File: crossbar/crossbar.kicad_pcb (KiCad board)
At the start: 2 copper layers, 57.2 x 57.2 mm, 22 parts, among them J1 Conn_01x16_Pin, J10 Conn_01x16_Pin, J11 Conn_01x16_Pin, J12 Conn_01x16_Pin, J13 Conn_01x16_Pin, J14 Conn_01x16_Pin, J15 Conn_01x16_Pin, J16 Conn_01x16_Pin, J17 Conn_01x16_Pin, J18 Conn_01x16_Pin, J19 Conn_01x04_Pin, J2 Conn_01x16_Socket, J20 Conn_01x04_Pin, J21 Conn_01x04_Socket, J22 Conn_01x04_Socket, J3 Conn_01x16_Pin, J4 Conn_01x16_Pin, J5 Conn_01x16_Pin, J6 Conn_01x16_Pin, J7 Conn_01x16_Pin, J8 Conn_01x16_Pin, J9 Conn_01x16_Pin

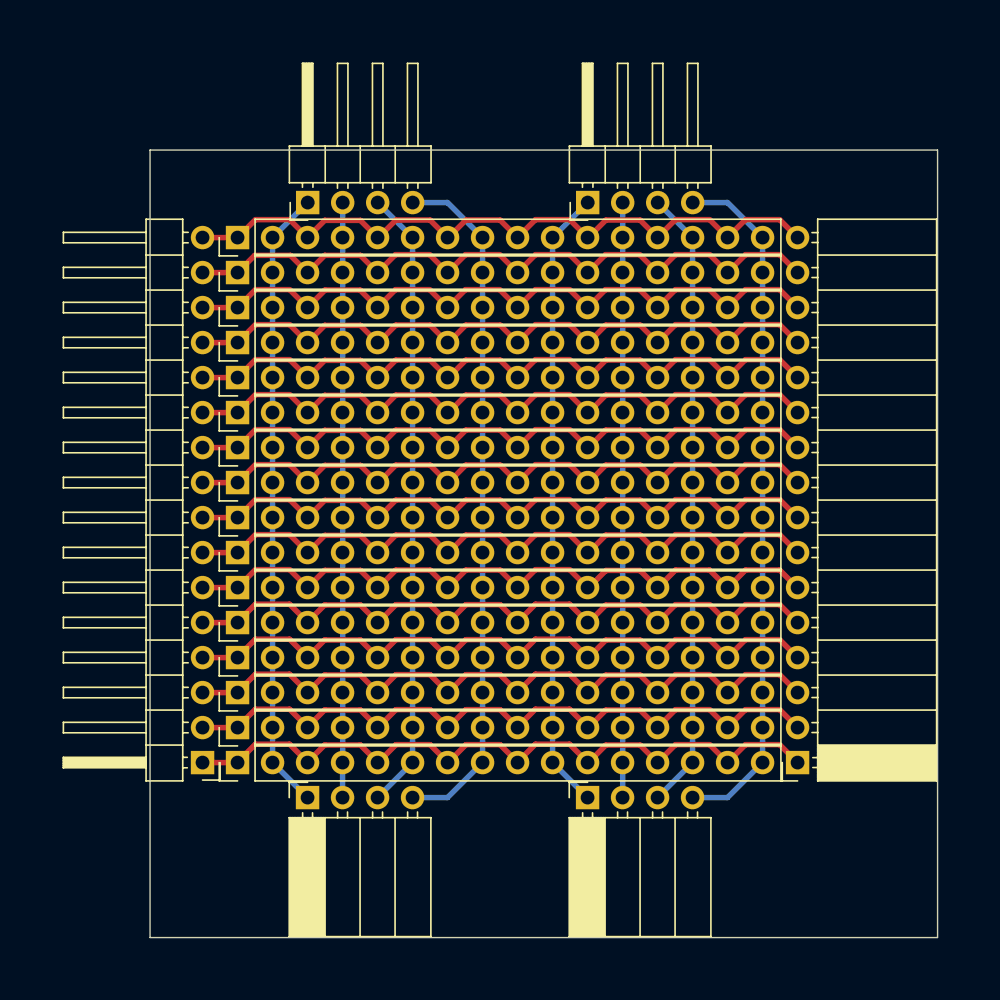
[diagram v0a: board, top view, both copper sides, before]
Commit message: crossbar & terminals
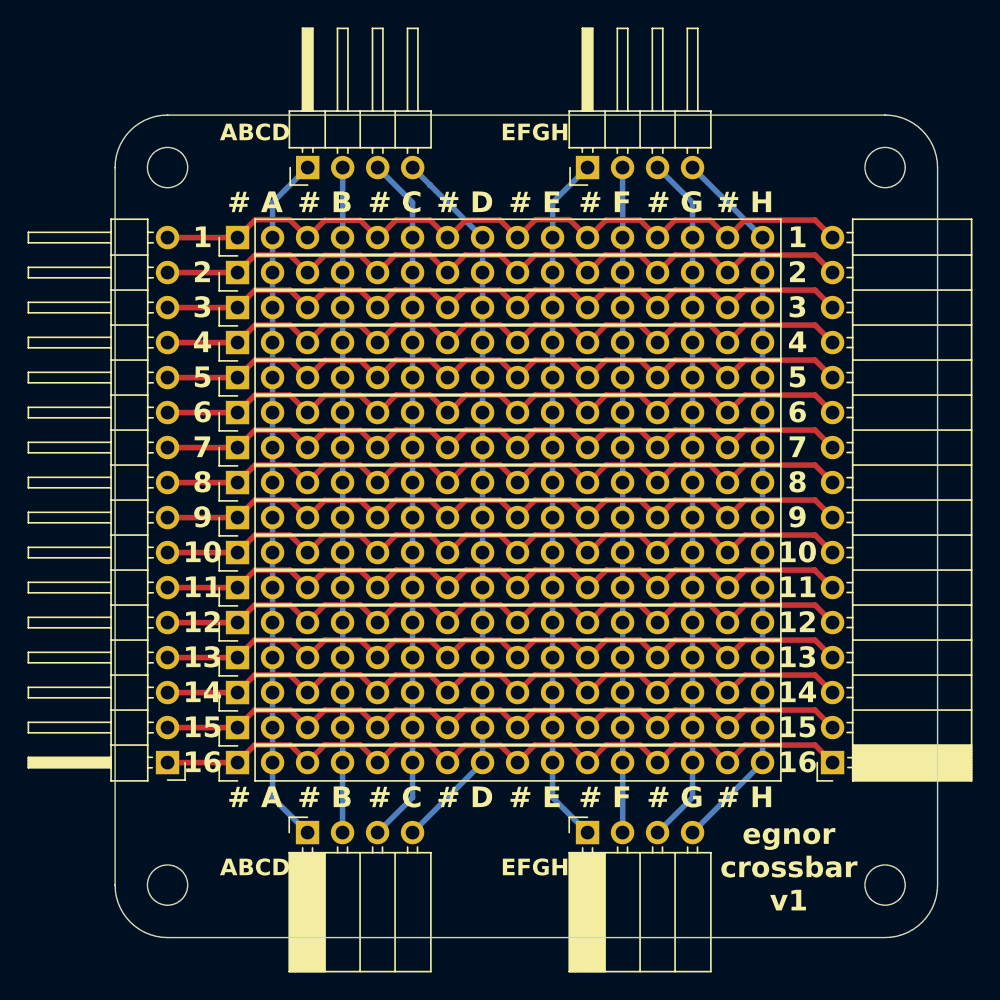
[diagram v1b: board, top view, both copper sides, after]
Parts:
- moved J20 2.54 mm to (170.2, 74.9)
- moved J1 2.54 mm to (139.7, 118.1)
- moved J2 2.54 mm to (188.0, 118.1)
- moved J19 2.54 mm to (149.9, 74.9)
- moved J21 2.54 mm to (149.9, 123.2)
- moved J22 2.54 mm to (170.2, 123.2)
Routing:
- net Net-(J10-Pin_12): track 43.2 -> 48.3 mm
- net Net-(J10-Pin_14): track 45.3 -> 50.4 mm
- net Net-(J10-Pin_2): track 45.3 -> 50.4 mm
- net Net-(J1-Pin_6): track 51.8 -> 56.8 mm
- net Net-(J10-Pin_6): track 45.3 -> 50.4 mm
- net Net-(J10-Pin_4): track 43.2 -> 48.2 mm
- net Net-(J10-Pin_10): track 45.3 -> 50.4 mm
- net Net-(J1-Pin_16): track 51.8 -> 56.8 mm
- net Net-(J1-Pin_9): track 51.8 -> 56.8 mm
- net Net-(J1-Pin_8): track 51.8 -> 56.7 mm
- net Net-(J1-Pin_11): track 51.8 -> 56.7 mm
- net Net-(J1-Pin_10): track 51.8 -> 56.7 mm
- net Net-(J1-Pin_7): track 51.8 -> 56.7 mm
- net Net-(J1-Pin_13): track 51.8 -> 56.7 mm
- net Net-(J1-Pin_12): track 51.8 -> 56.7 mm
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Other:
- board size 57.2 x 57.2 mm -> 59.7 x 59.7 mm
- board text added: "# A"
- board text added: "# B"
- board text added: "# C"
- board text added: "# D"
- board text added: "# E"
- board text added: "# F"
- board text added: "# G"
- board text added: "# H"
- board text added: "1"
- board text added: "10"
- board text added: "11"
- board text added: "12"
- board text added: "13"
- board text added: "14"
- board text added: "15"
- board text added: "16"
- board text added: "2"
- board text added: "3"
- board text added: "4"
- board text added: "5"
- board text added: "6"
- board text added: "7"
- board text added: "8"
- board text added: "9"
- board text added: "ABCD"
- board text added: "EFGH"
- board text added: "egnor crossbar v1"
